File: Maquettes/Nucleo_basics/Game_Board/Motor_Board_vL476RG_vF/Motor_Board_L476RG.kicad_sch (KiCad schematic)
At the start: 43 parts, among them CON1 MikroE-Accelero, CON2 MikroE-nRF-S-module, J1 Speed_R, J10 Morpho_Gauche, J11 Morpho_Droite, J12 LED_1, J13 LED_2, J14 LED_3, J15 LED_4, J17 I2C_Visu, J18 I2C_EXT, J19 GND_reg, J2 Speed_L, J20 3.3V_reg, J21 MOT_R, J22 MOT_L, J23 D_IN_OUT, J3 Line_R, J4 Line_C, J5 Line_L, J6 US_Sensor, J7 Servo, J8 BAT_IN, J9 TC74A2-TempI2C, SW1 SW_1, SW2 SW_2, U1 MCP9700-Temp, U2 LM7805_TO220, U3 SN754410NE

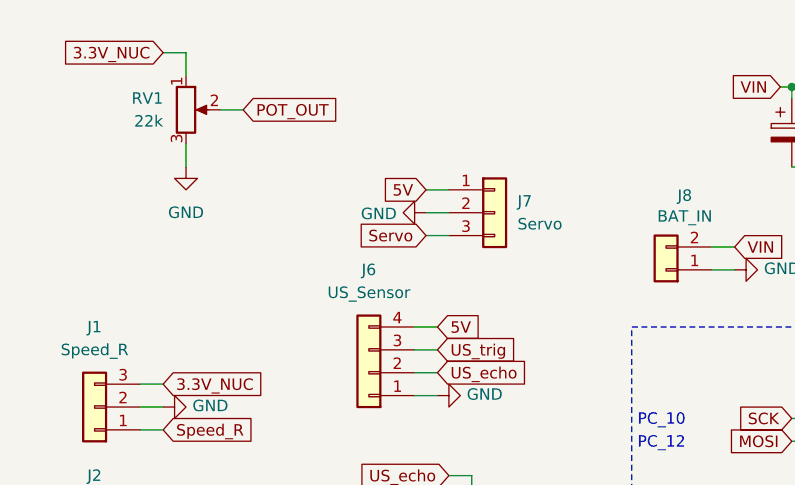
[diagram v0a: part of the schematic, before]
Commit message: Update Robot and Lighting Diagram boards
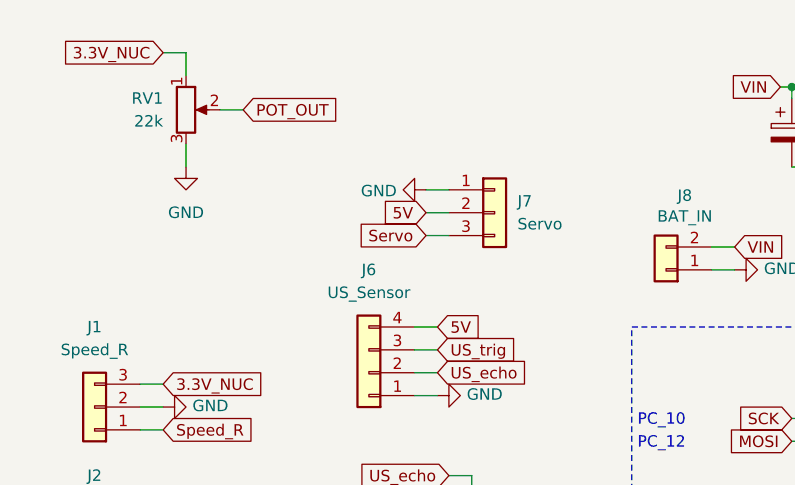
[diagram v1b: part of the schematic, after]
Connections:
- net 5V: now also J7.2 (Pin_2); no longer J7.1 (Pin_1)
- net GND: now also J7.1 (Pin_1); no longer J7.2 (Pin_2)
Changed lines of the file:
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@@
 	(global_label "5V"
 		(shape input)
-		(at 55.88 30.48 180)
+		(at 55.88 33.02 180)
 		(effects
 			(font
@@
 		)
 		(property "Intersheetrefs" "${INTERSHEET_REFS}"
-			(at 55.88 30.48 0)
+			(at 55.88 33.02 0)
 			(effects
 				(font
@@
 	(symbol
 		(lib_id "power:GND")
-		(at 55.88 33.02 270)
+		(at 55.88 30.48 270)
 		(unit 1)
 		(exclude_from_sim no)
@@
 		(dnp no)
 		(property "Reference" "#PWR09"
-			(at 49.53 33.02 0)
+			(at 49.53 30.48 0)
 			(effects
 				(font
@@
 		)
 		(property "Value" "GND"
-			(at 52.6288 33.147 90)
+			(at 52.6288 30.607 90)
 			(effects
 				(font
@@
 		)
 		(property "Footprint" ""
-			(at 55.88 33.02 0)
+			(at 55.88 30.48 0)
 			(effects
 				(font
@@
 		)
 		(property "Datasheet" ""
-			(at 55.88 33.02 0)
+			(at 55.88 30.48 0)
 			(effects
 				(font
@@
 		)
 		(property "Description" ""
-			(at 55.88 33.02 0)
+			(at 55.88 30.48 0)
 			(effects
 				(font
